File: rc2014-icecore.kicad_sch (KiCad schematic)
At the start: 19 parts, among them J1 Conn_01x39, J2 Conn_01x10, J3 Conn_02x25_Odd_Even, U1 LM1117-3.3, U2 SN74CB3T3245, U3 SN74CB3T3245, U4 SN74CB3T3245, U5 SN74CB3T3245, U6 SN74CB3T3245

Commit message: Further Kicad 6 updates
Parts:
- U1: symbol rc2014-icecore-rescue:LM1117-3.3 -> Regulator_Linear:LM1117-3.3
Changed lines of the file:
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@@
     (pin "1")
   )
-  (symbol (lib_id "rc2014-icecore-rescue:LM1117-3.3") (at 284.48 55.88 0) (unit 1)
+  (symbol (lib_id "Regulator_Linear:LM1117-3.3") (at 284.48 55.88 0) (unit 1)
     (in_bom yes) (on_board yes)
     (property "Reference" "U1" (id 0) (at 280.67 52.705 0))
@@
       (effects (font (size 1.27 1.27)) hide)
     )
-    (property "Datasheet" "" (id 3) (at 284.48 55.88 0)
+    (property "Datasheet" "http://www.ti.com/lit/ds/symlink/lm1117.pdf" (id 3) (at 284.48 55.88 0)
       (effects (font (size 1.27 1.27)) hide)
     )

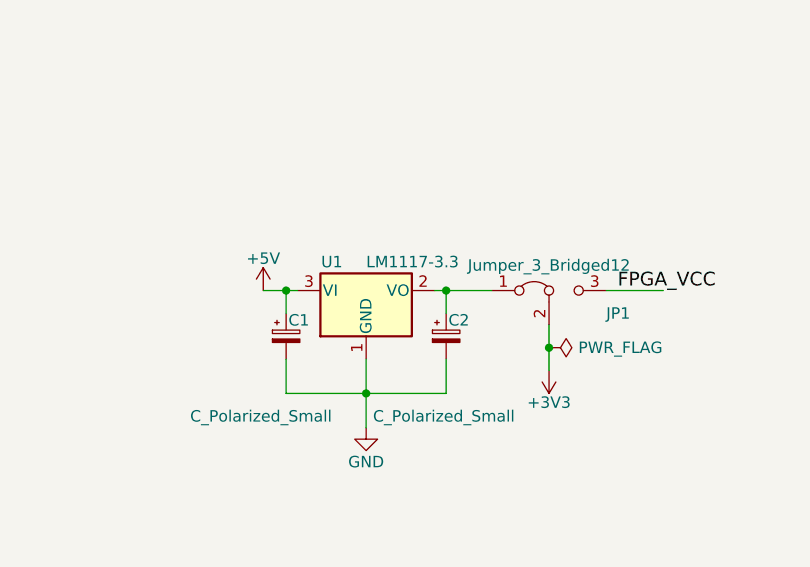
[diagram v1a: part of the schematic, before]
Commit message: Update to kicad 7
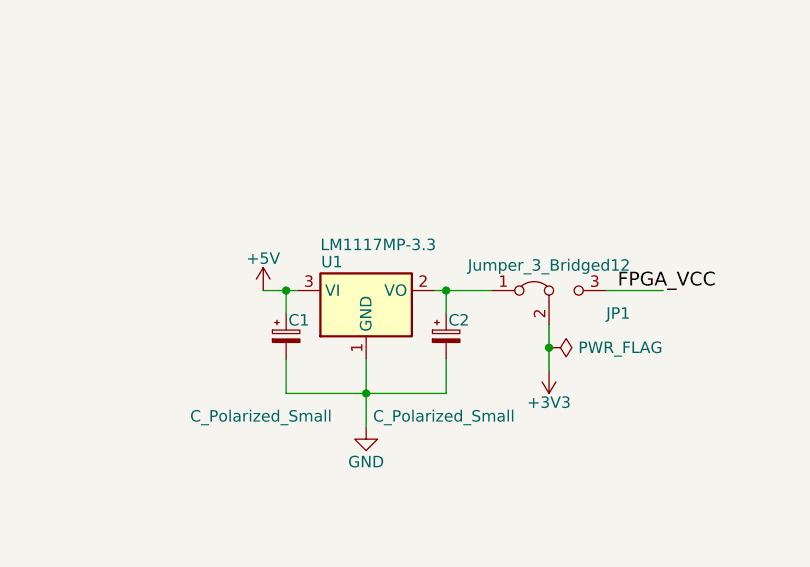
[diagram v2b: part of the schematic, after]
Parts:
- U1: value LM1117-3.3 -> LM1117MP-3.3; symbol Regulator_Linear:LM1117-3.3 -> Regulator_Linear:LM1117MP-3.3
